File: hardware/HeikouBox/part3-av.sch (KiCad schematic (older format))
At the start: 92 parts, among them J301 DB15_Female_HighDensity_Mount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, J302 AudioJack3_SwitchTR, Q301 MMBT3904, Q302 MMBT3904, Q303 MMBT3904, Q304 MMBT3904, Q305 MMBT3904, Q306 MMBT3904, Q307 MMBT3904

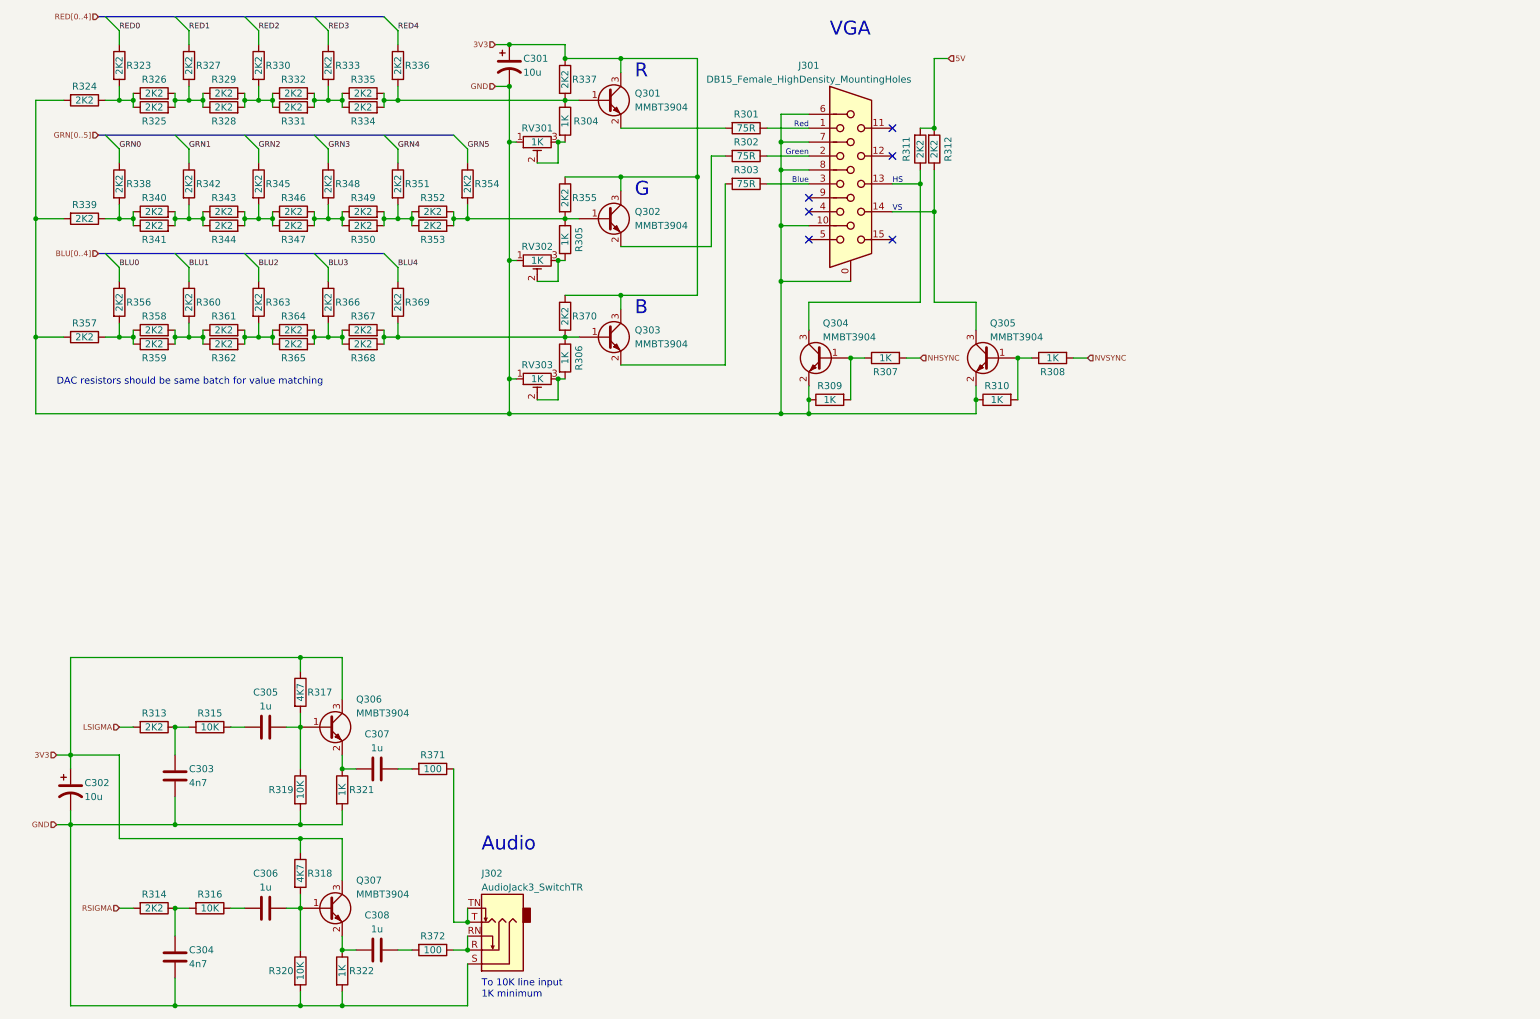
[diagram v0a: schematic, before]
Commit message: Mainboard v0.1 PCB ready for export
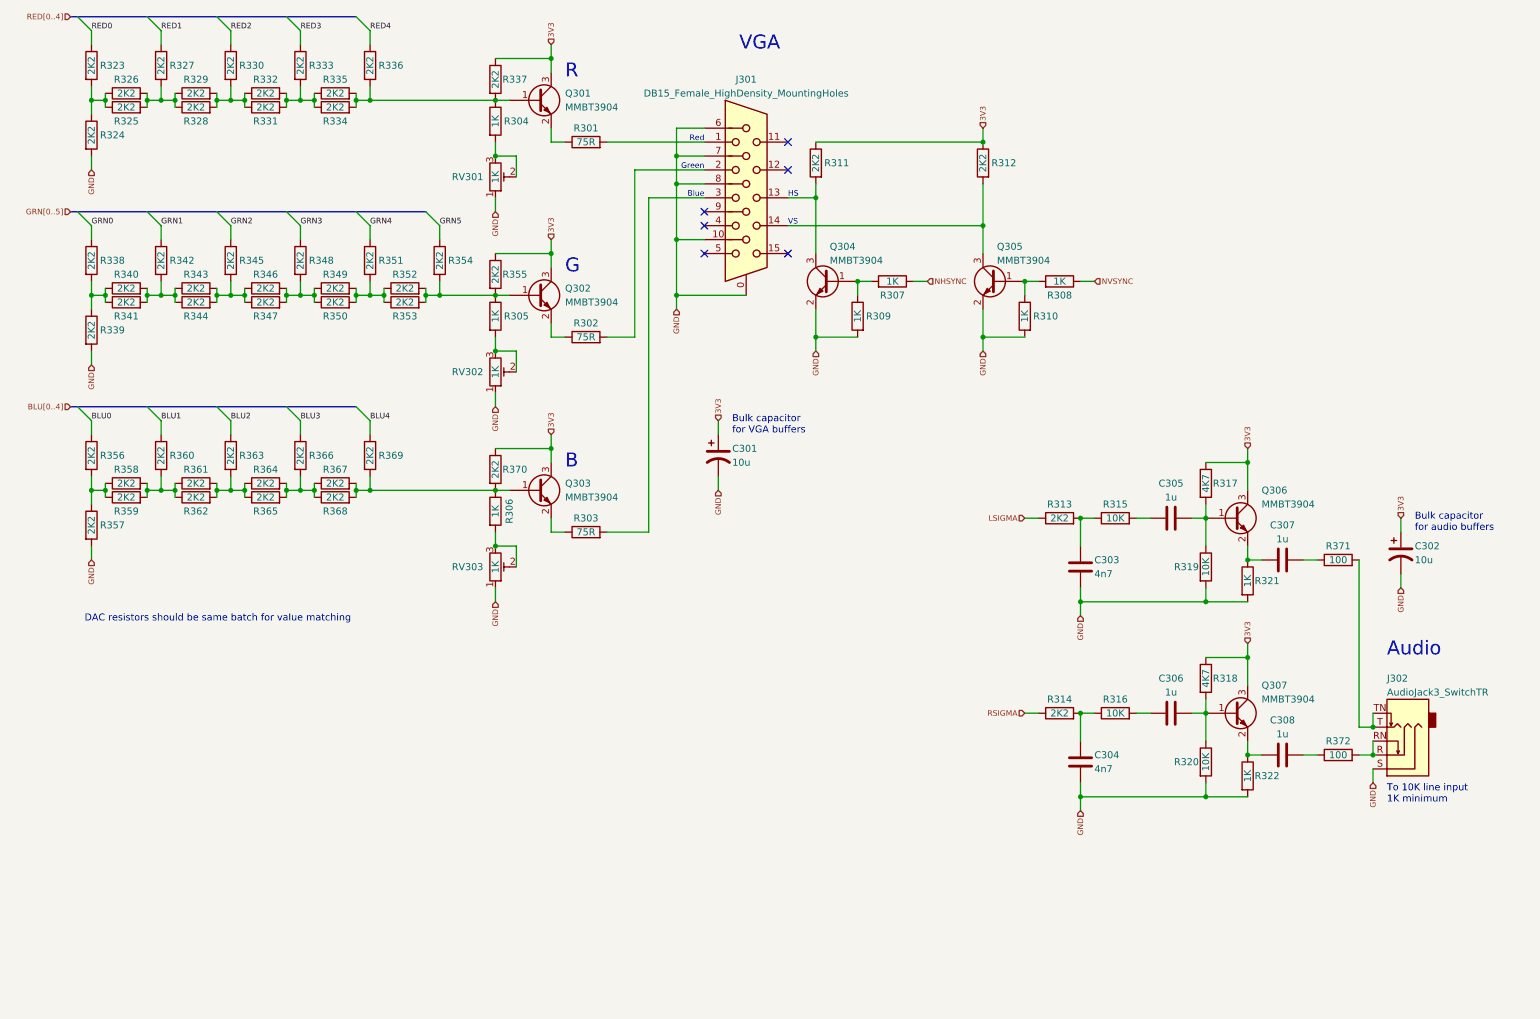
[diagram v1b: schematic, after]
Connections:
- net 3V3: now also R311.1, R312.1
- net GND: now also R309.2, R310.2; no longer R309.1, R310.1
- net LSIGMA: now also R313.1; no longer R313.2
- net NHSYNC: now also R307.1; no longer R307.2
- net NVSYNC: now also R308.1; no longer R308.2
- net RSIGMA: now also R314.1; no longer R314.2
- net at Q307.2 (E), R322.1: now also C308.1; no longer C308.2
- net at Q307.1 (B), R318.2, R320.1: now also C306.2; no longer C306.1
- net at Q306.1 (B), R317.2, R319.1: now also C305.2; no longer C305.1
- net at R315.1: now also C303.1, R313.2; no longer C305.2
- net at Q306.2 (E), R321.1: now also C307.1; no longer C307.2
- net at R371.2: now also J302.T, J302.TN; no longer C307.1
- net at J301.14, Q305.3 (C): now also R312.2; no longer R312.1
- net at J301.13, Q304.3 (C): now also R311.2; no longer R311.1
- net at R302.1: now also Q302.2 (E); no longer J301.2
- net at R302.2: now also J301.2; no longer Q302.2 (E)
- net at R303.1: now also Q303.2 (E); no longer J301.3
- net at R303.2: now also J301.3; no longer Q303.2 (E)
- net at Q301.2 (E): now also R301.1; no longer R301.2
- net at J301.1: now also R301.2; no longer R301.1
- net at R316.1: now also C304.1, R314.2; no longer C306.2
- net at R372.2: now also J302.R, J302.RN; no longer C308.1
- removed net 5V: R311.2, R312.2
- new net: C305.1, R315.2
- new net: C307.2, R371.1
- new net: Q304.1 (B), R307.2, R309.1
- new net: Q305.1 (B), R308.2, R310.1
- new net: C306.1, R316.2
- new net: C308.2, R372.1
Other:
- note added: "Bulk capacitor\nfor VGA buffers"
- note added: "Bulk capacitor\nfor audio buffers"
- moved on the sheet: C301, C302, C303, C304, C305, C306, C307, C308, J301, J302, Q301, Q302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
